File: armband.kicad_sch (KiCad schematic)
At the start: 14 parts, among them IC1 QSMP-1570, SW1 EVP-BB2A9B000, SW2 EVP-BB2A9B000

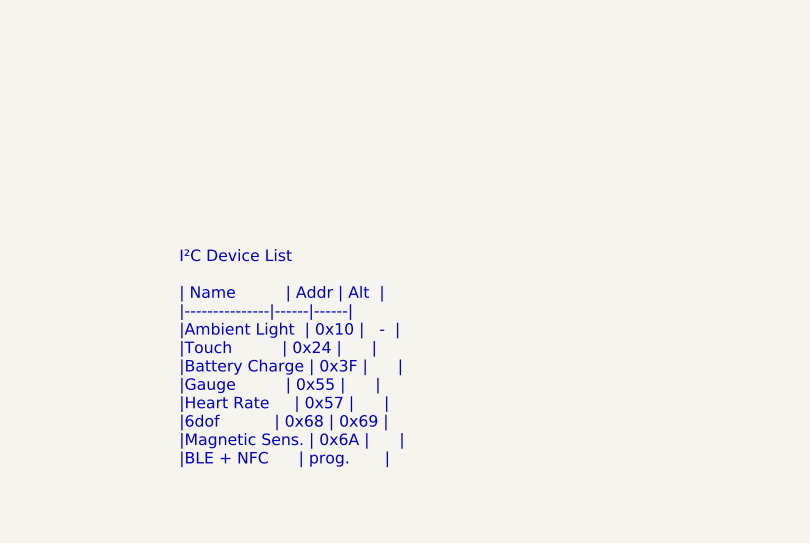
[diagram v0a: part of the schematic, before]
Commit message: Update 3d models
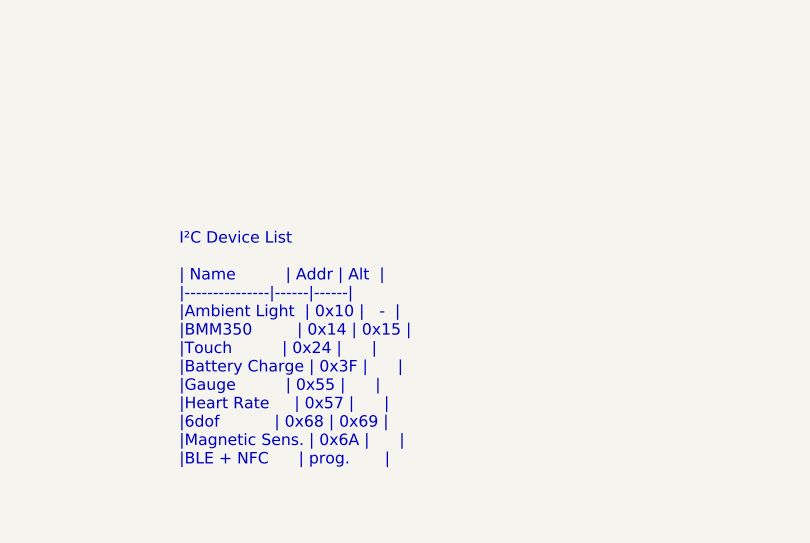
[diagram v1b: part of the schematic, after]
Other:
- note added: "I²C Device List | Name | Addr | Alt | |---------------|------|------| |Ambient Light | 0x10 | - | |BMM350 | 0x14 | 0x15 | |Touch | 0x24 | | |Battery Charge | 0x3F | | |Gauge | 0x55 | | |Heart Rate | 0x57 | | |6dof | 0x68 | 0x69 | |Magnetic Sens. | 0x6A | | |BLE + NFC | prog. |"
- note removed: "I²C Device List | Name | Addr | Alt | |---------------|------|------| |Ambient Light | 0x10 | - | |Touch | 0x24 | | |Battery Charge | 0x3F | | |Gauge | 0x55 | | |Heart Rate | 0x57 | | |6dof | 0x68 | 0x69 | |Magnetic Sens. | 0x6A | | |BLE + NFC | prog. |"
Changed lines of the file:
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@@
     (effects (font (size 1.27 1.27)) (justify left bottom))
   )
-  (text "I²C Device List\n\n| Name          | Addr | Alt  |\n|---------------|------|------|\n|Ambient Light  | 0x10 |   -  |\n|Touch          | 0x24 |      |\n|Battery Charge | 0x3F |      |  \n|Gauge          | 0x55 |      |  \n|Heart Rate     | 0x57 |      |\n|6dof           | 0x68 | 0x69 |\n|Magnetic Sens. | 0x6A |      |\n|BLE + NFC      | prog.       |"
+  (text "I²C Device List\n\n| Name          | Addr | Alt  |\n|---------------|------|------|\n|Ambient Light  | 0x10 |   -  |\n|BMM350         | 0x14 | 0x15 |\n|Touch          | 0x24 |      |\n|Battery Charge | 0x3F |      |  \n|Gauge          | 0x55 |      |  \n|Heart Rate     | 0x57 |      |\n|6dof           | 0x68 | 0x69 |\n|Magnetic Sens. | 0x6A |      |\n|BLE + NFC      | prog.       |"
     (at 254 279.4 0)
     (effects (font (face "Cascadia Mono") (size 1.27 1.27)) (justify left bottom))

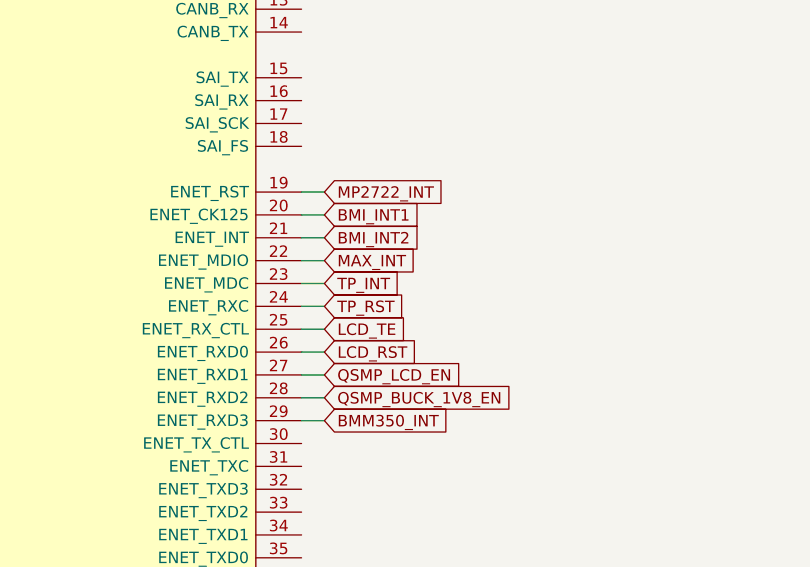
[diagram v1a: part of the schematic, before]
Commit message: progressed layout
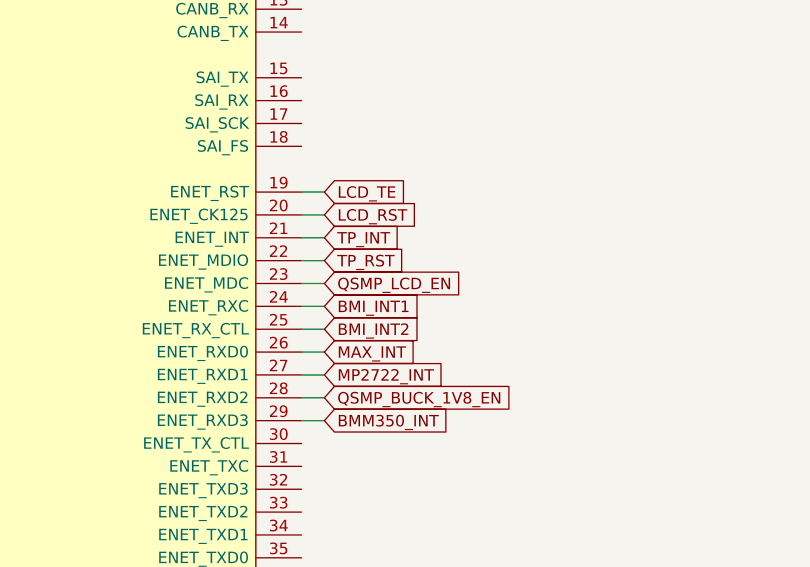
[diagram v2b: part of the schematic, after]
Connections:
- net BMI_INT1: now also IC1.24 (ENET_RXC); no longer IC1.20 (ENET_CK125)
- net BMI_INT2: now also IC1.25 (ENET_RX_CTL); no longer IC1.21 (ENET_INT)
- net LCD_RST: now also IC1.20 (ENET_CK125); no longer IC1.26 (ENET_RXD0)
- net LCD_TE: now also IC1.19 (ENET_RST); no longer IC1.25 (ENET_RX_CTL)
- net MAX_INT: now also IC1.26 (ENET_RXD0); no longer IC1.22 (ENET_MDIO)
- net MP2722_INT: now also IC1.27 (ENET_RXD1); no longer IC1.19 (ENET_RST)
- net QSMP_LCD_EN: now also IC1.23 (ENET_MDC); no longer IC1.27 (ENET_RXD1)
- net TP_INT: now also IC1.21 (ENET_INT); no longer IC1.23 (ENET_MDC)
- net TP_RST: now also IC1.22 (ENET_MDIO); no longer IC1.24 (ENET_RXC)
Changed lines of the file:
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@@
     )
   )
-  (global_label "BMI_INT2" (shape input) (at 236.22 139.7 0) (fields_autoplaced)
-    (effects (font (size 1.27 1.27)) (justify left))
-    (property "Intersheetrefs" "${INTERSHEET_REFS}" (at 247.532 139.7 0)
+  (global_label "BMI_INT2" (shape input) (at 236.22 149.86 0) (fields_autoplaced)
+    (effects (font (size 1.27 1.27)) (justify left))
+    (property "Intersheetrefs" "${INTERSHEET_REFS}" (at 247.532 149.86 0)
       (effects (font (size 1.27 1.27)) (justify left) hide)
     )
@@
     )
   )
-  (global_label "TP_RST" (shape input) (at 236.22 147.32 0) (fields_autoplaced)
-    (effects (font (size 1.27 1.27)) (justify left))
-    (property "Intersheetrefs" "${INTERSHEET_REFS}" (at 245.7781 147.32 0)
+  (global_label "TP_RST" (shape input) (at 236.22 142.24 0) (fields_autoplaced)
+    (effects (font (size 1.27 1.27)) (justify left))
+    (property "Intersheetrefs" "${INTERSHEET_REFS}" (at 245.7781 142.24 0)
       (effects (font (size 1.27 1.27)) (justify left) hide)
     )
@@
     )
   )
-  (global_label "QSMP_LCD_EN" (shape input) (at 236.22 154.94 0) (fields_autoplaced)
-    (effects (font (size 1.27 1.27)) (justify left))
-    (property "Intersheetrefs" "${INTERSHEET_REFS}" (at 252.37 154.94 0)
+  (global_label "QSMP_LCD_EN" (shape input) (at 236.22 144.78 0) (fields_autoplaced)
+    (effects (font (size 1.27 1.27)) (justify left))
+    (property "Intersheetrefs" "${INTERSHEET_REFS}" (at 252.37 144.78 0)
       (effects (font (size 1.27 1.27)) (justify left) hide)
     )
@@
     )
   )
-  (global_label "MP2722_INT" (shape input) (at 236.22 134.62 0) (fields_autoplaced)
-    (effects (font (size 1.27 1.27)) (justify left))
-    (property "Intersheetrefs" "${INTERSHEET_REFS}" (at 250.5557 134.62 0)
+  (global_label "MP2722_INT" (shape input) (at 236.22 154.94 0) (fields_autoplaced)
+    (effects (font (size 1.27 1.27)) (justify left))
+    (property "Intersheetrefs" "${INTERSHEET_REFS}" (at 250.5557 154.94 0)
       (effects (font (size 1.27 1.27)) (justify left) hide)
     )
@@
     )
   )
-  (global_label "MAX_INT" (shape input) (at 236.22 142.24 0) (fields_autoplaced)
-    (effects (font (size 1.27 1.27)) (justify left))
-    (property "Intersheetrefs" "${INTERSHEET_REFS}" (at 246.7458 142.24 0)
+  (global_label "MAX_INT" (shape input) (at 236.22 152.4 0) (fields_autoplaced)
+    (effects (font (size 1.27 1.27)) (justify left))
+    (property "Intersheetrefs" "${INTERSHEET_REFS}" (at 246.7458 152.4 0)
       (effects (font (size 1.27 1.27)) (justify left) hide)
     )
@@
     )
   )
-  (global_label "BMI_INT1" (shape input) (at 236.22 137.16 0) (fields_autoplaced)
-    (effects (font (size 1.27 1.27)) (justify left))
-    (property "Intersheetrefs" "${INTERSHEET_REFS}" (at 247.532 137.16 0)
+  (global_label "BMI_INT1" (shape input) (at 236.22 147.32 0) (fields_autoplaced)
+    (effects (font (size 1.27 1.27)) (justify left))
+    (property "Intersheetrefs" "${INTERSHEET_REFS}" (at 247.532 147.32 0)
       (effects (font (size 1.27 1.27)) (justify left) hide)
     )
@@
     )
   )
-  (global_label "LCD_TE" (shape input) (at 236.22 149.86 0) (fields_autoplaced)
-    (effects (font (size 1.27 1.27)) (justify left))
-    (property "Intersheetrefs" "${INTERSHEET_REFS}" (at 245.7781 149.86 0)
+  (global_label "LCD_TE" (shape input) (at 236.22 134.62 0) (fields_autoplaced)
+    (effects (font (size 1.27 1.27)) (justify left))
+    (property "Intersheetrefs" "${INTERSHEET_REFS}" (at 245.7781 134.62 0)
       (effects (font (size 1.27 1.27)) (justify left) hide)
     )
@@
     )
   )
-  (global_label "LCD_RST" (shape input) (at 236.22 152.4 0) (fields_autoplaced)
-    (effects (font (size 1.27 1.27)) (justify left))
-    (property "Intersheetrefs" "${INTERSHEET_REFS}" (at 247.1086 152.4 0)
+  (global_label "LCD_RST" (shape input) (at 236.22 137.16 0) (fields_autoplaced)
+    (effects (font (size 1.27 1.27)) (justify left))
+    (property "Intersheetrefs" "${INTERSHEET_REFS}" (at 247.1086 137.16 0)
       (effects (font (size 1.27 1.27)) (justify left) hide)
     )
@@
     )
   )
-  (global_label "TP_INT" (shape input) (at 236.22 144.78 0) (fields_autoplaced)
-    (effects (font (size 1.27 1.27)) (justify left))
-    (property "Intersheetrefs" "${INTERSHEET_REFS}" (at 245.2339 144.78 0)
-      (effects (font (size 1.27 1.27)) (justify left) hide)
-    )
+  (global_label "TP_INT" (shape input) (at 236.22 139.7 0) (fields_autoplaced)
+    (effects (font (size 1.27 1.27)) (justify left))
+    (property "Intersheetrefs" "${INTERSHEET_REFS}" (at 245.2339 139.7 0)
+      (effects (font (size 1.27 1.27)) (justify left) hide)
+    )
